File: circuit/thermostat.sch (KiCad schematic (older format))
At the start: 13 parts

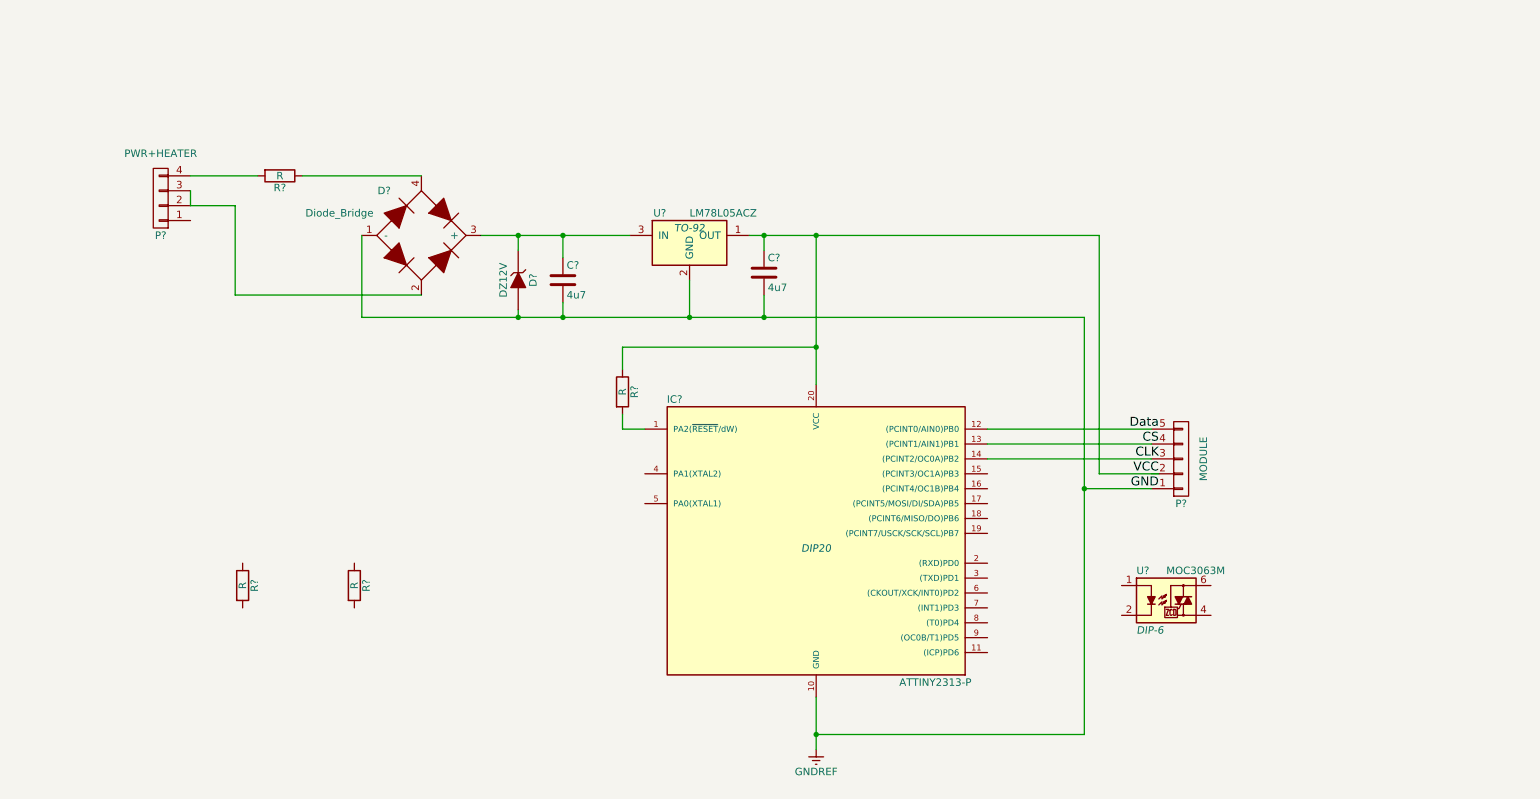
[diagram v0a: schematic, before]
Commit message: Still in progress
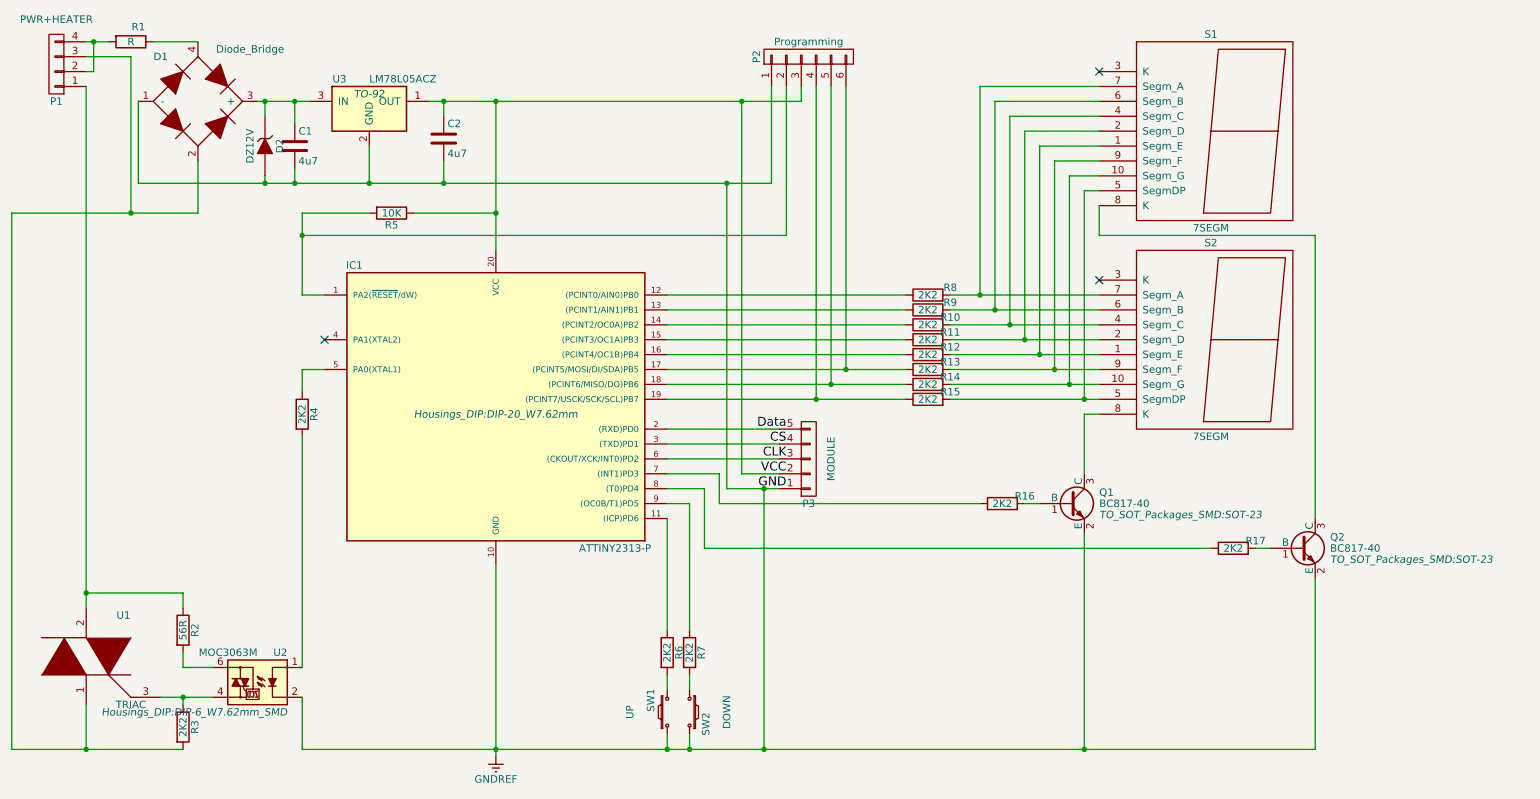
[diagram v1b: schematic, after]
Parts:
- added P2: Programming, Socket_Strips:Socket_Strip_Straight_1x06_Pitch2.54mm, symbol CONN_01X06
- added Q1, Q2: BC817-40, TO_SOT_Packages_SMD:SOT-23, symbol BC817-40
- added R10, R11, R12, R13, R14, R15, R16, R17, R3, R4, R6, R9: 2K2, Resistors_SMD:R_0805_HandSoldering, symbol R
- added R2: 56R, Resistors_SMD:R_0805_HandSoldering, symbol R
- added S1, S2: 7SEGM, symbol 7SEGM
- added SW1: UP, symbol SW_PUSH_SMALL_H
- added SW2: DOWN, symbol SW_PUSH_SMALL_H
- added U1: TRIAC, Socket_Strips:Socket_Strip_Angled_1x03_Pitch2.54mm, symbol TRIAC
- C1, C2: renamed from C?; footprint (none) -> Capacitors_SMD:C_0805_HandSoldering
- D1: renamed from D?; footprint (none) -> Diodes_ThroughHole:Diode_Bridge_15.7x15.7
- D2: renamed from D?; footprint (none) -> Diodes_SMD:D_0805
- IC1: renamed from IC?; footprint DIP20 -> Housings_DIP:DIP-20_W7.62mm
- P1: renamed from P?; footprint (none) -> Socket_Strips:Socket_Strip_Angled_1x04_Pitch2.54mm
- P3: renamed from P?; footprint (none) -> Socket_Strips:Socket_Strip_Angled_1x05_Pitch2.54mm
- R1: renamed from R?; footprint (none) -> Resistors_SMD:R_0805_HandSoldering
- R5: renamed from R?; value R -> 10K; footprint (none) -> Resistors_SMD:R_0805_HandSoldering
- R7, R8: renamed from R?; value R -> 2K2; footprint (none) -> Resistors_SMD:R_0805_HandSoldering
- U2: renamed from U?; footprint DIP-6 -> Housings_DIP:DIP-6_W7.62mm_SMD
- gave numbers to parts that had none: 1
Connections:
- net GNDREF: now also U2.2, P2.1 (P1), Q1.2 (E), Q2.2 (E), SW1.1, SW2.2
- net VCC: no longer C2.1, IC1.20 (VCC), R5.1, U3.1 (OUT)
- net at P3.2 (P2): now also C2.1, IC1.20 (VCC), R5.1, U3.1 (OUT), P2.3 (P3)
- net at P3.3 (P3): now also IC1.6 ((CKOUT/XCK/INT0)PD2); no longer IC1.14 ((PCINT2/OC0A)PB2)
- net at P3.4 (P4): now also IC1.3 ((TXD)PD1); no longer IC1.13 ((PCINT1/AIN1)PB1)
- net at P3.5 (P5): now also IC1.2 ((RXD)PD0); no longer IC1.12 ((PCINT0/AIN0)PB0)
- net at IC1.1 (PA2(~RESET~/dW)), R5.2: now also P2.2 (P2)
- net at IC1.11 ((ICP)PD6): now also R6.1
- net at IC1.15 ((PCINT3/OC1A)PB3): now also R11.1
- net at IC1.16 ((PCINT4/OC1B)PB4): now also R12.1
- net at IC1.17 ((PCINT5/MOSI/DI/SDA)PB5): now also P2.6 (P6), R13.1
- net at IC1.18 ((PCINT6/MISO/DO)PB6): now also P2.5 (P5), R14.1
- net at IC1.19 ((PCINT7/USCK/SCK/SCL)PB7): now also P2.4 (P4), R15.1
- net at IC1.5 (PA0(XTAL1)): now also R4.1
- net at IC1.7 ((INT1)PD3): now also R16.1
- net at IC1.8 ((T0)PD4): now also R17.1
- net at IC1.9 ((OC0B/T1)PD5): now also R7.1
- net at P1.4 (P4), R1.2: now also P1.2 (P2)
- net at D1.2, P1.3 (P3): now also R3.2, U1.1; no longer P1.2 (P2)
- net at P1.1 (P1): now also R2.1, U1.2
- net at U2.1: now also R4.2
- net at U2.4: now also R3.1, U1.3
- net at U2.6: now also R2.2
- net at R8.1: now also IC1.12 ((PCINT0/AIN0)PB0)
- net at R8.2: now also S1.7 (Segm_A), S2.7 (Segm_A)
- net at R7.2: now also SW2.1
- new net: IC1.13 ((PCINT1/AIN1)PB1), R9.1
- new net: IC1.14 ((PCINT2/OC0A)PB2), R10.1
- new net: R12.2, S1.1 (Segm_E), S2.1 (Segm_E)
- new net: R14.2, S1.10 (Segm_G), S2.10 (Segm_G)
- new net: R11.2, S1.2 (Segm_D), S2.2 (Segm_D)
- new net: R10.2, S1.4 (Segm_C), S2.4 (Segm_C)
- new net: R15.2, S1.5 (SegmDP), S2.5 (SegmDP)
- new net: R9.2, S1.6 (Segm_B), S2.6 (Segm_B)
- new net: Q2.3 (C), S1.8 (K)
- new net: R13.2, S1.9 (Segm_F), S2.9 (Segm_F)
- new net: Q1.3 (C), S2.8 (K)
- new net: Q1.1 (B), R16.2
- new net: Q2.1 (B), R17.2
- new net: R6.2, SW1.2
- no-connect marks 0 -> 3
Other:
- moved on the sheet: C1, C2, D1, D2, IC1, P1, P3, R1, R5, R7, R8, U2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

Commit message: Finished schematic
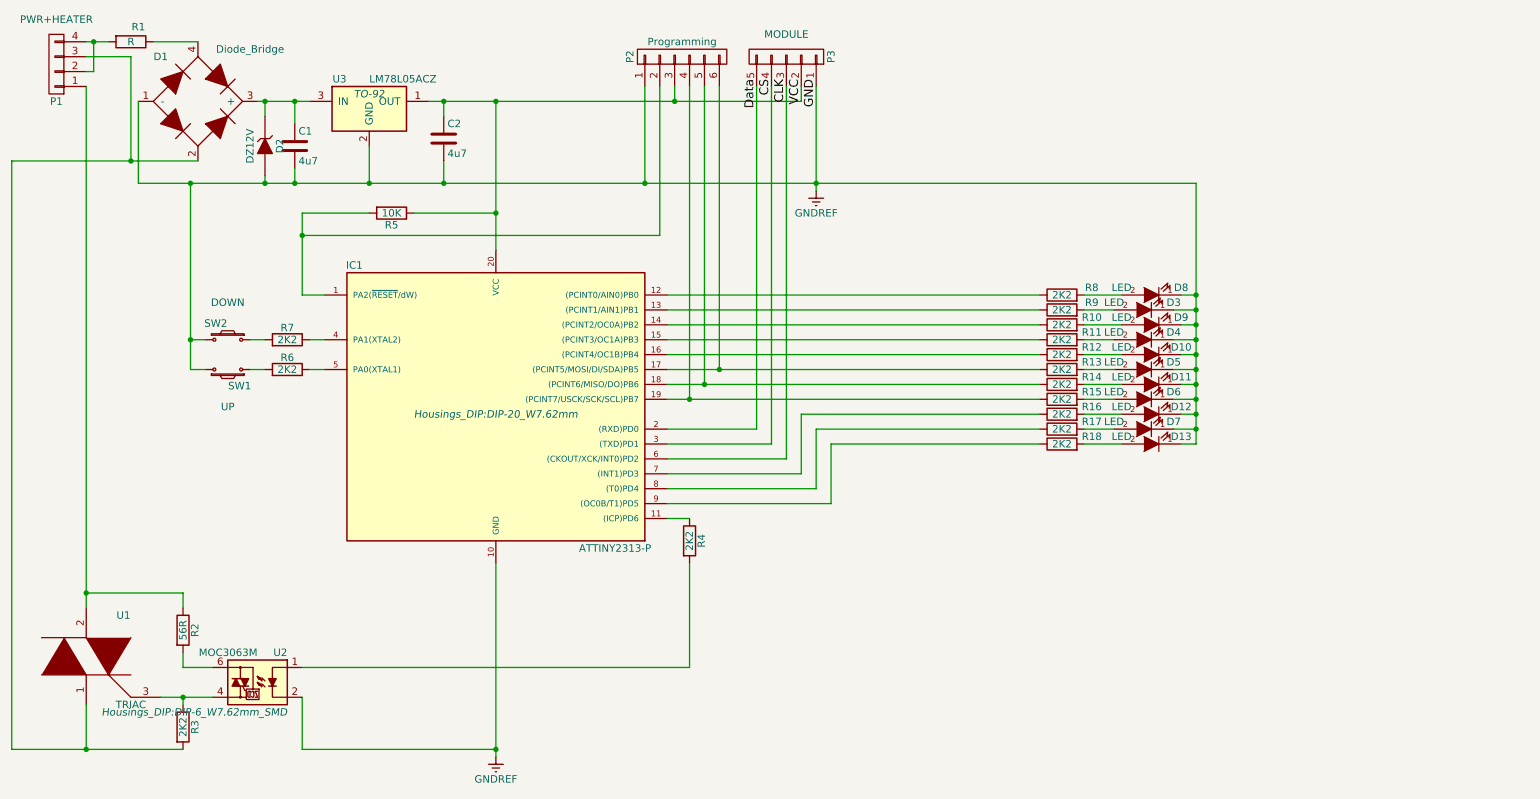
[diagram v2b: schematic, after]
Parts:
- removed Q1, Q2: BC817-40, TO_SOT_Packages_SMD:SOT-23, symbol BC817-40
- removed S1, S2: 7SEGM, symbol 7SEGM
- added D10, D11, D12, D13, D3, D4, D5, D6, D7, D8, D9: LED, Socket_Strips:Socket_Strip_Straight_1x02_Pitch2.54mm, symbol LED
- added R18: 2K2, Resistors_SMD:R_0805_HandSoldering, symbol R
- SW1, SW2: footprint (none) -> custom_sw:Micro_sw_1
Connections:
- net GNDREF: now also D10.1 (K), D11.1 (K), D12.1 (K), D13.1 (K), D3.1 (K), D4.1 (K), D5.1 (K), D6.1 (K), D7.1 (K), D8.1 (K), D9.1 (K)
- net at IC1.11 ((ICP)PD6): now also R4.1; no longer R6.1
- net at IC1.4 (PA1(XTAL2)): now also R7.1
- net at IC1.5 (PA0(XTAL1)): now also R6.1; no longer R4.1
- net at IC1.9 ((OC0B/T1)PD5): now also R18.1; no longer R7.1
- net at R8.2: now also D8.2 (A)
- net at R12.2: now also D10.2 (A)
- net at R14.2: now also D11.2 (A)
- net at R11.2: now also D4.2 (A)
- net at R10.2: now also D9.2 (A)
- net at R15.2: now also D6.2 (A)
- net at R9.2: now also D3.2 (A)
- net at R13.2: now also D5.2 (A)
- net at R16.2: now also D12.2 (A)
- net at R17.2: now also D7.2 (A)
- new net: D13.2 (A), R18.2
- no-connect marks 3 -> 0
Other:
- moved on the sheet: P2, P3, R10, R11, R12, R13, R14, R15, R4, R6, R7, R8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
